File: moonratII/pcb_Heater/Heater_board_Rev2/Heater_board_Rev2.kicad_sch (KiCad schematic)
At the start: 11 parts, among them J10 Conn_02x05_Odd_Even, J11 Screw_Terminal_01x02, J9 Screw_Terminal_01x06

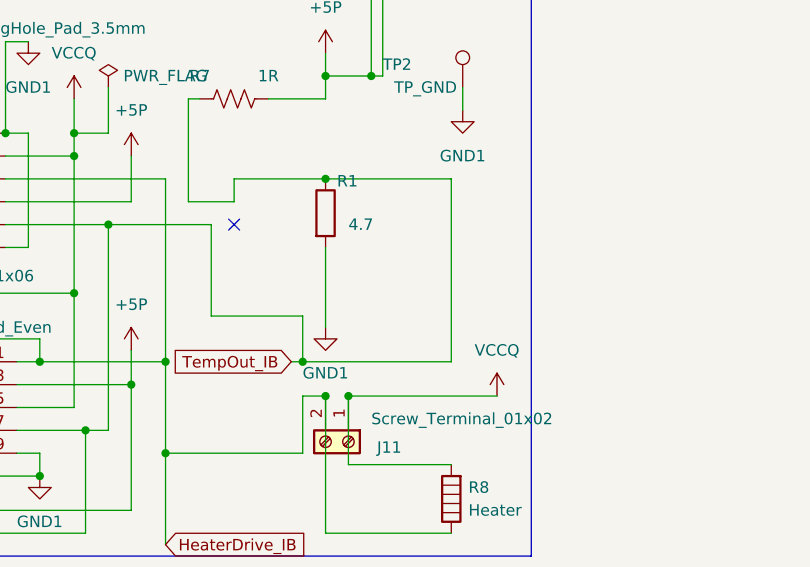
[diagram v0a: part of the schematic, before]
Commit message: Added Dallas One to heater board.
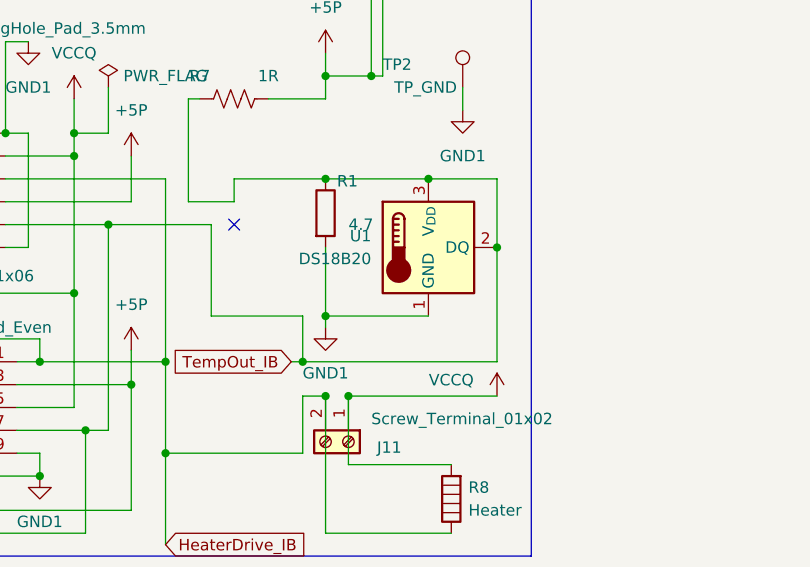
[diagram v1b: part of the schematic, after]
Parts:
- added U1: DS18B20, Package_TO_SOT_THT:TO-92_Inline, symbol Sensor_Temperature:DS18B20
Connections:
- net GND1: now also U1.1 (GND)
- net TempOut_IB: now also U1.2 (DQ), U1.3 (V_{DD})
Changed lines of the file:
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@@
+	)
+	(junction
+		(at 234.95 111.76)
+		(diameter 0)
+		(color 0 0 0 0)
 	)
 	(junction
@@
 	)
 	(junction
+		(at 254 119.38)
+		(diameter 0)
+		(color 0 0 0 0)
+	)
+	(junction
 		(at 203.2 132.08)
 		(diameter 0)
@@
 	)
 	(junction
+		(at 234.95 127)
+		(diameter 0)
+		(color 0 0 0 0)
+	)
+	(junction
 		(at 210.82 116.84)
+		(diameter 0)
+		(color 0 0 0 0)
+	)
+	(junction
+		(at 246.38 111.76)
 		(diameter 0)
 		(color 0 0 0 0)
@@
 		(color 0 0 0 0)
 	)
-	(junction
-		(at 234.95 111.76)
-		(diameter 0)
-		(color 0 0 0 0)
-	)
 	(no_connect
 		(at 224.79 116.84)
@@
 	(wire
 		(pts
+			(xy 254 119.38) (xy 254 132.08)
+		)
+		(stroke
+			(width 0)
+			(type default)
+		)
+	)
+	(wire
+		(pts
 			(xy 181.61 124.46) (xy 207.01 124.46)
 		)
@@
 	(wire
 		(pts
+			(xy 234.95 127) (xy 246.38 127)
+		)
+		(stroke
+			(width 0)
+			(type default)
+		)
+	)
+	(wire
+		(pts
 			(xy 181.61 148.59) (xy 213.36 148.59)
 		)
@@
 	(wire
 		(pts
-			(xy 232.41 132.08) (xy 248.92 132.08)
+			(xy 232.41 132.08) (xy 254 132.08)
 		)
 		(stroke
@@
 	(wire
 		(pts
-			(xy 234.95 119.38) (xy 234.95 128.27)
-		)
-		(stroke
-			(width 0)
-			(type default)
-		)
-	)
-	(wire
-		(pts
 			(xy 210.82 116.84) (xy 222.25 116.84)
 		)
@@
 	(wire
 		(pts
+			(xy 234.95 127) (xy 234.95 128.27)
+		)
+		(stroke
+			(width 0)
+			(type default)
+		)
+	)
+	(wire
+		(pts
 			(xy 246.38 81.915) (xy 246.38 83.185)
 		)
@@
 	(wire
 		(pts
-			(xy 234.95 111.76) (xy 248.92 111.76)
-		)
-		(stroke
-			(width 0)
-			(type default)
-		)
-	)
-	(wire
-		(pts
 			(xy 224.79 114.3) (xy 224.79 111.76)
 		)
@@
 	(wire
 		(pts
-			(xy 248.92 111.76) (xy 248.92 132.08)
+			(xy 254 111.76) (xy 254 119.38)
+		)
+		(stroke
+			(width 0)
+			(type default)
+		)
+	)
+	(wire
+		(pts
+			(xy 234.95 119.38) (xy 234.95 127)
 		)
 		(stroke
@@
 	(wire
 		(pts
+			(xy 246.38 111.76) (xy 254 111.76)
+		)
+		(stroke
+			(width 0)
+			(type default)
+		)
+	)
+	(wire
+		(pts
 			(xy 203.2 132.08) (xy 217.17 132.08)
 		)
@@
 		(pts
 			(xy 207.01 137.16) (xy 200.66 137.16)
+		)
+		(stroke
+			(width 0)
+			(type default)
+		)
+	)
+	(wire
+		(pts
+			(xy 234.95 111.76) (xy 246.38 111.76)
 		)
 		(stroke
@@
 		(on_board yes)
 		(dnp no)
-		(fields_autoplaced yes)
 		(property "Reference" "#PWR017"
 			(at 254 139.7 0)
@@
 		)
 		(property "Value" "VCCQ"
-			(at 254 130.81 0)
+			(at 248.92 134.112 0)
 			(effects
 				(font
@@
 					(unit 1)
 				)
+			)
+		)
+	)
+	(symbol
+		(lib_id "Sensor_Temperature:DS18B20")
+		(at 246.38 119.38 0)
+		(unit 1)
+		(exclude_from_sim no)
+		(in_bom yes)
+		(on_board yes)
+		(dnp no)
+		(fields_autoplaced yes)
+		(property "Reference" "U1"
+			(at 240.03 118.1099 0)
+			(effects
+				(font
+					(size 1.27 1.27)
+				)
+				(justify right)
+			)
+		)
+		(property "Value" "DS18B20"
+			(at 240.03 120.6499 0)
+			(effects
+				(font
+					(size 1.27 1.27)
+				)
+				(justify right)
+			)
+		)
+		(property "Footprint" "Package_TO_SOT_THT:TO-92_Inline"
+			(at 220.98 125.73 0)
+			(effects
+				(font
+					(size 1.27 1.27)
+				)
+				(hide yes)
+			)
+		)
+		(property "Datasheet" "http://datasheets.maximintegrated.com/en/ds/DS18B20.pdf"
+			(at 242.57 113.03 0)
+			(effects
+				(font
+					(size 1.27 1.27)
+				)
+				(hide yes)
+			)
+		)
+		(property "Description" "Programmable Resolution 1-Wire Digital Thermometer TO-92"
+			(at 246.38 119.38 0)
+			(effects
+				(font
+					(size 1.27 1.27)
+				)
+				(hide yes)
+			)
+		)
+		(pin "1"
+		)
+		(pin "3"
+		)
+		(pin "2"
+		)
+		(instances
+			(project ""
+				(path "/9ef5effe-cb46-4a9a-bbbe-a65ab44b9e67"
+					(reference "U1")
+					(unit 1)
+				)
